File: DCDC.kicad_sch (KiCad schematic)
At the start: 25 parts, among them U5 LM76005RNPR

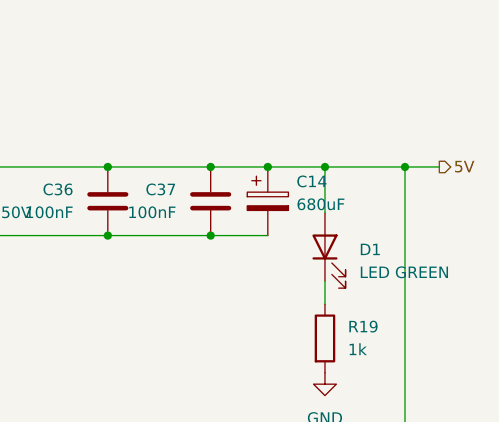
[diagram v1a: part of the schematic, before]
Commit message: Finish v0.2 PCB and DRC
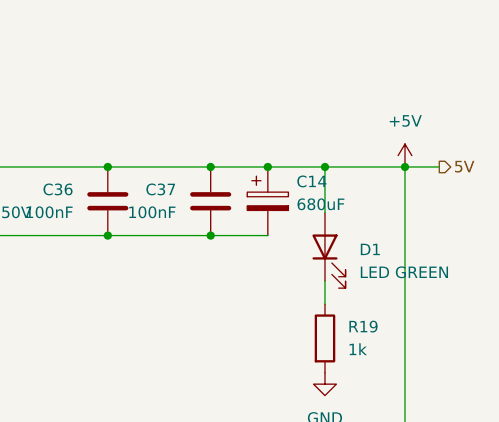
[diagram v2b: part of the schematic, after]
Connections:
- net 5V renamed +5V
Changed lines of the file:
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@@
+	)
+	(symbol
+		(lib_id "power:+5V")
+		(at 346.71 115.57 0)
+		(unit 1)
+		(exclude_from_sim no)
+		(in_bom yes)
+		(on_board yes)
+		(dnp no)
+		(fields_autoplaced yes)
+		(property "Reference" "#PWR018"
+			(at 346.71 119.38 0)
+			(effects
+				(font
+					(size 1.27 1.27)
+				)
+				(hide yes)
+			)
+		)
+		(property "Value" "+5V"
+			(at 346.71 110.49 0)
+			(effects
+				(font
+					(size 1.27 1.27)
+				)
+			)
+		)
+		(property "Footprint" ""
+			(at 346.71 115.57 0)
+			(effects
+				(font
+					(size 1.27 1.27)
+				)
+				(hide yes)
+			)
+		)
+		(property "Datasheet" ""
+			(at 346.71 115.57 0)
+			(effects
+				(font
+					(size 1.27 1.27)
+				)
+				(hide yes)
+			)
+		)
+		(property "Description" "Power symbol creates a global label with name \"+5V\""
+			(at 346.71 115.57 0)
+			(effects
+				(font
+					(size 1.27 1.27)
+				)
+				(hide yes)
+			)
+		)
+		(pin "1"
+		)
+		(instances
+			(project ""
+				(path "/e12e8a63-1d1b-4736-9aba-a87a258b2b11/a934a33d-5c23-43ea-a123-a23c10f76236"
+					(reference "#PWR018")
+					(unit 1)
+				)
+			)
+		)
 	)
 	(symbol

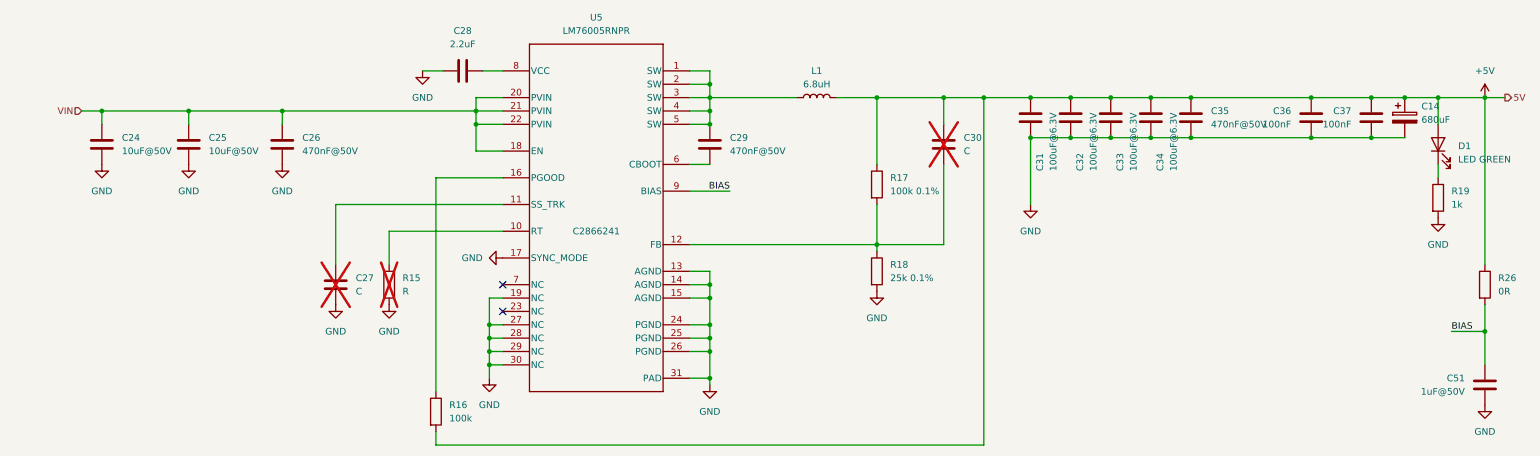
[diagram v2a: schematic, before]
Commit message: Restructured v0.1 for easier worktree use
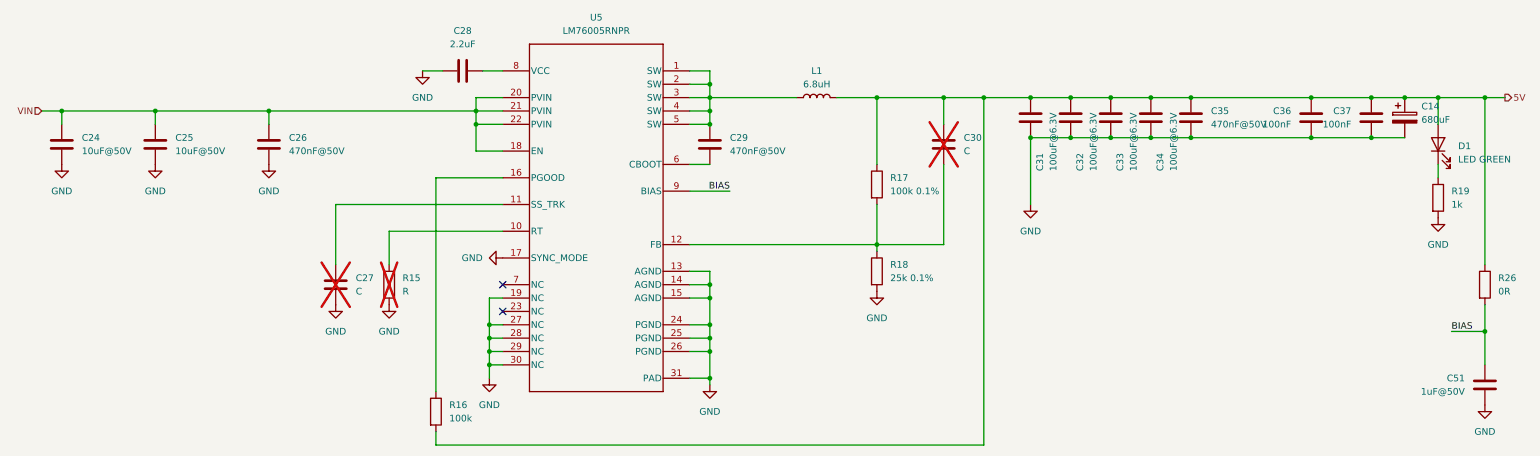
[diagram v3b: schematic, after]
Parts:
- U5: JLC (none) -> C2866241; LCSC Part # C2866241 -> (none)
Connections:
- net +5V renamed 5V
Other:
- moved on the sheet: C24, C25, C26
